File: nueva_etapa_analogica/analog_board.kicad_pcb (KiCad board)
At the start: 2 copper layers, 31.5 x 50.1 mm, 44 parts, among them J101 Conn_01x02, J102 Conn_01x03, J103 Conn_01x03, J104 Conn_01x03, J105 Conn_01x03, J106 Conn_01x03, J107 Conn_01x03, J108 Conn_01x03, J109 Conn_01x03, J110 Conn_01x03, J111 Conn_01x02, U101 MAX4522CSE+, U102 TLV3544, U103 CPC1017N, U104 CPC1017N, U105 CPC1017N, U106 CPC1017N

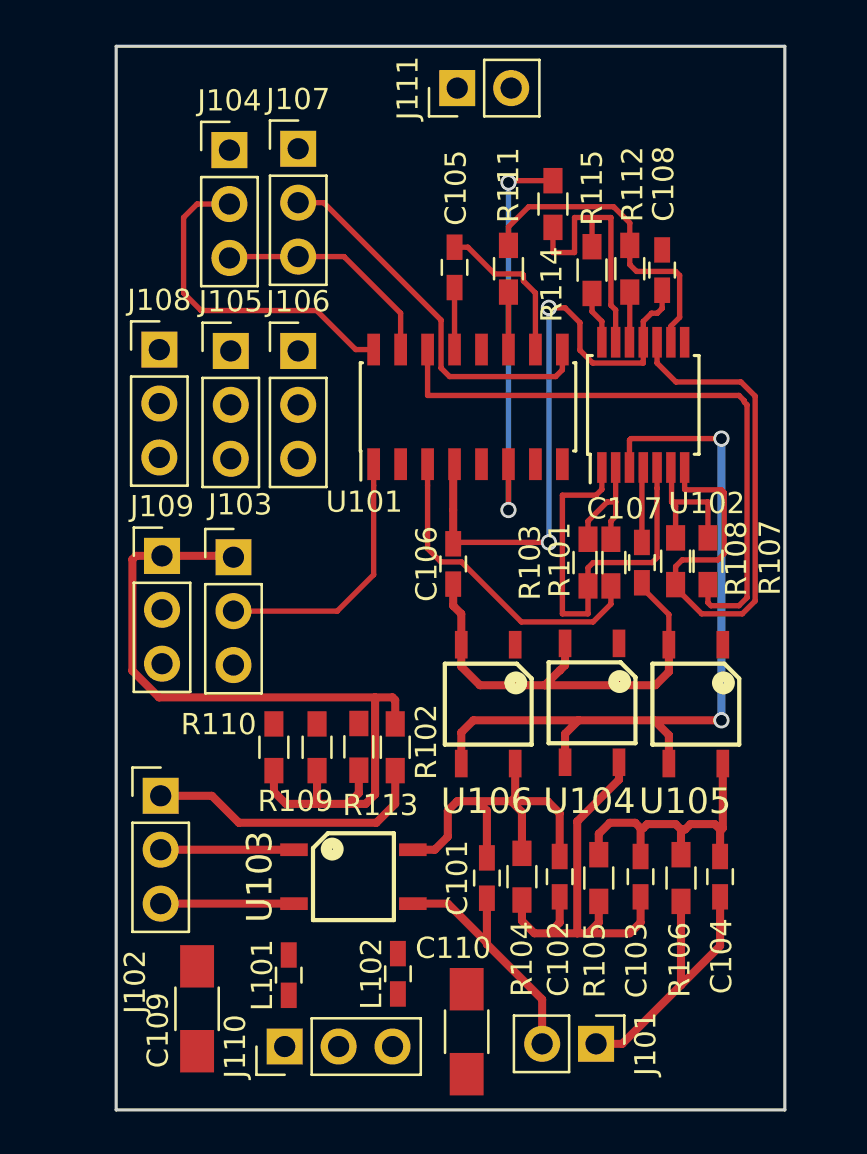
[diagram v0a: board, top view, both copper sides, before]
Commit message: Finished with routing.
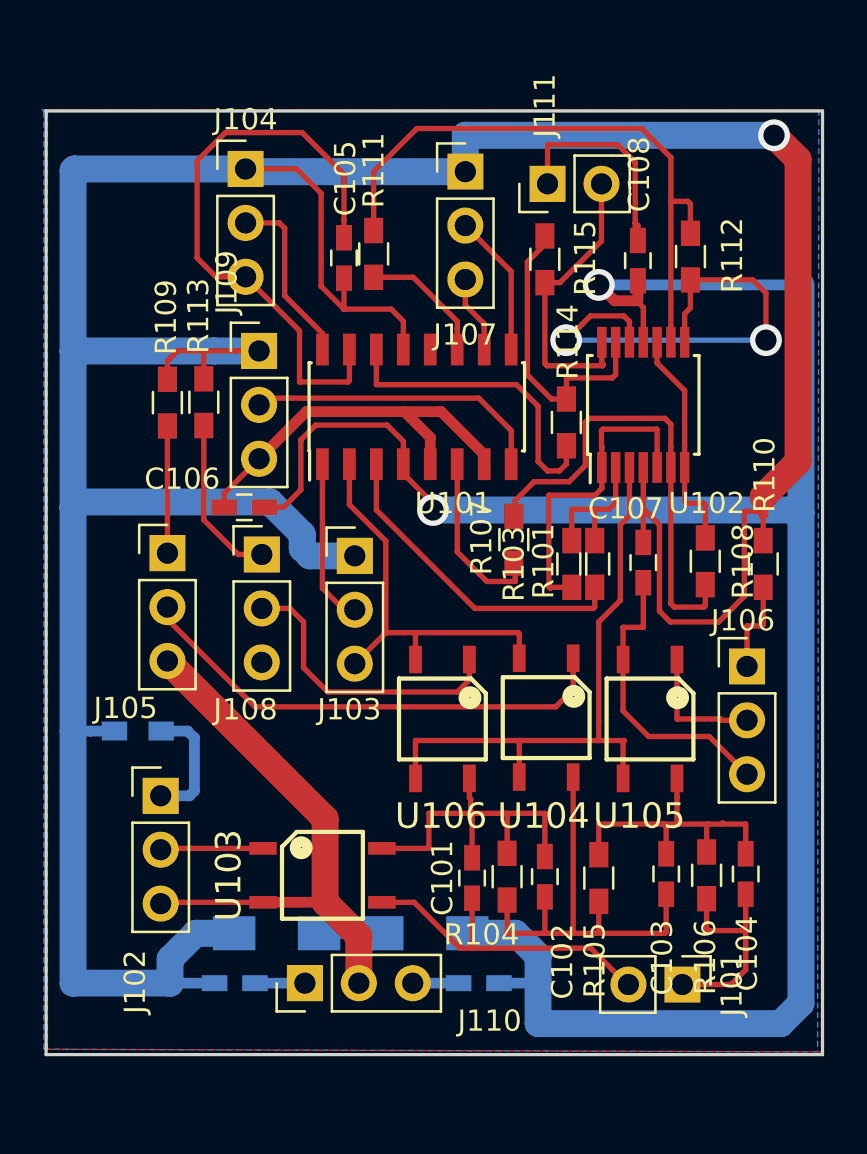
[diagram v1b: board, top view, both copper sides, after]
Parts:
- C109, C110, L101, L102, R102: moved to B.Cu
- moved J106 25.8 mm to (142.2, 97.8)
- moved R110 24.6 mm to (143.0, 93.0), turned to 90 degrees
- moved R113 17.8 mm to (116.6, 85.3), turned to 90 degrees
- moved R109 17.7 mm to (114.9, 85.4), turned to 90 degrees
- moved R102 12.2 mm to (113.5, 100.8), turned to 180 degrees
- moved J108 10.8 mm to (119.4, 92.5)
- moved J109 10.7 mm to (119.3, 82.9)
- moved R114 10.3 mm to (133.7, 86.3), turned to 90 degrees
- moved C106 10.2 mm to (118.6, 90.3), turned to 0 degrees
- moved J105 9.98 mm to (114.9, 92.5)
- moved R107 9.20 mm to (131.3, 91.8)
- moved J107 7.95 mm to (129.0, 74.5)
- moved R111 6.39 mm to (124.7, 78.4)
- moved J111 6.20 mm to (132.8, 75.1)
- moved J103 5.72 mm to (123.8, 92.6)
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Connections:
- U101 pad 14: Net-(R107-Pad1) -> Net-(R114-Pad1)
- U101 pad 6: Net-(R114-Pad1) -> Net-(R107-Pad1)
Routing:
- net VDD: track 44.8 -> 170.9 mm, vias 0 -> 1
- net GND: track 60.3 -> 137.5 mm
- net VSS: track 29.6 -> 101.1 mm
- net Net-(J105-Pad2): track 0.00 -> 23.1 mm
- net Net-(R107-Pad1): track 29.4 -> 8.69 mm
- net Net-(R112-Pad1): track 2.37 -> 23.0 mm, vias 0 -> 2
- net Net-(R108-Pad1): track 29.8 -> 10.6 mm
- net Net-(R107-Pad2): track 6.50 -> 21.8 mm
- net Net-(J109-Pad2): track 0.00 -> 14.2 mm
- net Net-(R111-Pad2): track 15.1 -> 29.3 mm
- net Net-(J108-Pad2): track 0.00 -> 13.9 mm
- net Net-(J107-Pad2): track 18.3 -> 6.73 mm
- net Net-(J111-Pad2): track 2.49 -> 13.9 mm
- net /Vatt: track 37.5 -> 28.6 mm, vias 2 -> 0
- net Net-(J108-Pad1): track 0.00 -> 7.85 mm
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- added copper zone on B.Cu, net GND
- added copper zone on F.Cu, net GND
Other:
- board size 31.5 x 50.1 mm -> 36.6 x 44.5 mm
- net class Default: via_dia 0.762 -> 1.5; via_drill 0.508 -> 1
